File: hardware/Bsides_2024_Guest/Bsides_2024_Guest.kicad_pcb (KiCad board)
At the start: 2 copper layers, 134.5 x 127.4 mm, 45 parts, among them J1 Conn_02x03_Odd_Even, J2 Battery, J3 Battery, J4 OLED, J5 Conn_01x05, J6 Conn_01x05, P1 USB_C_Plug_USB2.0, Q1 DMG3415U-7, SW1 ON, SW2 RESET, SW3 BOOT, SW4 RESET, SW6 RESET, U1 ESP32-C6-WROOM-1U-N4, U2 AP2112K-3.3

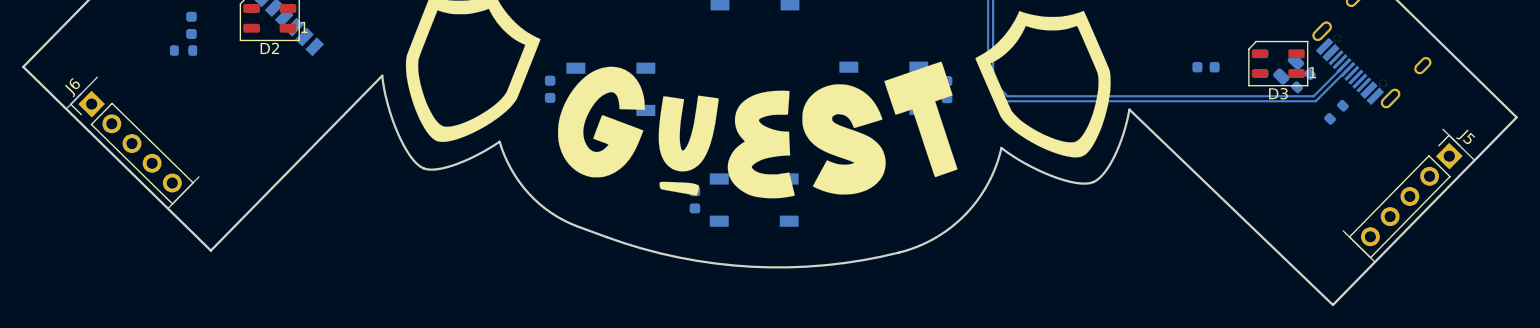
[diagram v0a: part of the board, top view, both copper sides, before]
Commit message: feat(Hw): Update PCB
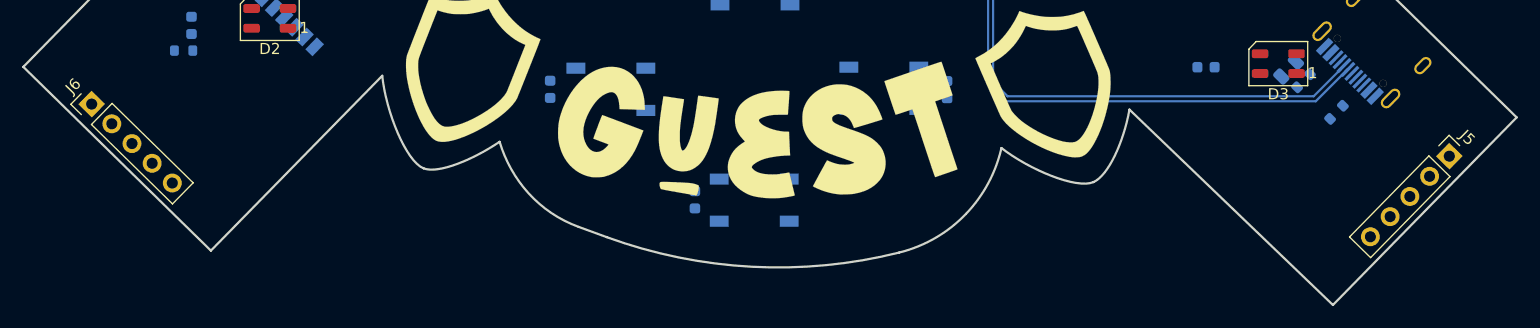
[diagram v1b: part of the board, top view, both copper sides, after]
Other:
- outline, holes or cut-outs redrawn
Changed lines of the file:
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@@
 		(fp_arc
 			(start -2.500001 3.299999)
-			(mid -2.449999 3.249997)
+			(mid -2.45 3.249996)
 			(end -2.4 3.300001)
 			(stroke
@@
 		(fp_arc
 			(start -2.500001 3.299999)
-			(mid -2.449999 3.249997)
+			(mid -2.45 3.249996)
 			(end -2.4 3.300001)
 			(stroke
@@
 		(fp_arc
 			(start -2.4 3.300001)
-			(mid -2.450001 3.349998)
+			(mid -2.45 3.349997)
 			(end -2.500001 3.299999)
 			(stroke
@@
 		(layer "Edge.Cuts")
 	)
-	(gr_line
-		(start 71.276522 144.729814)
-		(end 74.075973 141.872705)
-		(stroke
-			(width 0.05)
-			(type default)
-		)
-		(layer "Edge.Cuts")
-	)
 	(gr_curve
 		(pts
@@
 		(layer "Edge.Cuts")
 	)
-	(gr_line
-		(start 188.961906 140.388346)
-		(end 186.104797 137.588895)
-		(stroke
-			(width 0.05)
-			(type default)
-		)
-		(layer "Edge.Cuts")
-	)
 	(gr_curve
 		(pts
@@
 		(layer "Edge.Cuts")
 	)
-	(gr_line
-		(start 192.750825 136.520175)
-		(end 188.961906 140.388346)
-		(stroke
-			(width 0.05)
-			(type default)
-		)
-		(layer "Edge.Cuts")
-	)
 	(gr_curve
 		(pts
@@
 	)
 	(gr_line
-		(start 176.202092 153.414868)
-		(end 179.991011 149.546697)
-		(stroke
-			(width 0.05)
-			(type default)
-		)
-		(layer "Edge.Cuts")
-	)
-	(gr_line
-		(start 58.25 131.97)
-		(end 62.118171 135.758919)
-		(stroke
-			(width 0.05)
-			(type default)
-		)
-		(layer "Edge.Cuts")
-	)
-	(gr_line
 		(start 58.25 131.97)
 		(end 75.144693 148.518733)
@@
 		(layer "Edge.Cuts")
 	)
-	(gr_line
-		(start 64.917622 132.90181)
-		(end 62.118171 135.758919)
-		(stroke
-			(width 0.05)
-			(type default)
-		)
-		(layer "Edge.Cuts")
-	)
 	(gr_curve
 		(pts
@@
 		(layer "Edge.Cuts")
 	)
-	(gr_line
-		(start 75.144693 148.518733)
-		(end 71.276522 144.729814)
-		(stroke
-			(width 0.05)
-			(type default)
-		)
-		(layer "Edge.Cuts")
-	)
 	(gr_curve
 		(pts
@@
 			(type default)
 		)
-		(layer "Edge.Cuts")
-	)
-	(gr_line
-		(start 177.133902 146.747246)
-		(end 179.991011 149.546697)
-		(stroke
-			(width 0.05)
-			(type default)
-		)
